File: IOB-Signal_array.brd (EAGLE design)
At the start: 106.7 x 104.1 mm, 104 parts

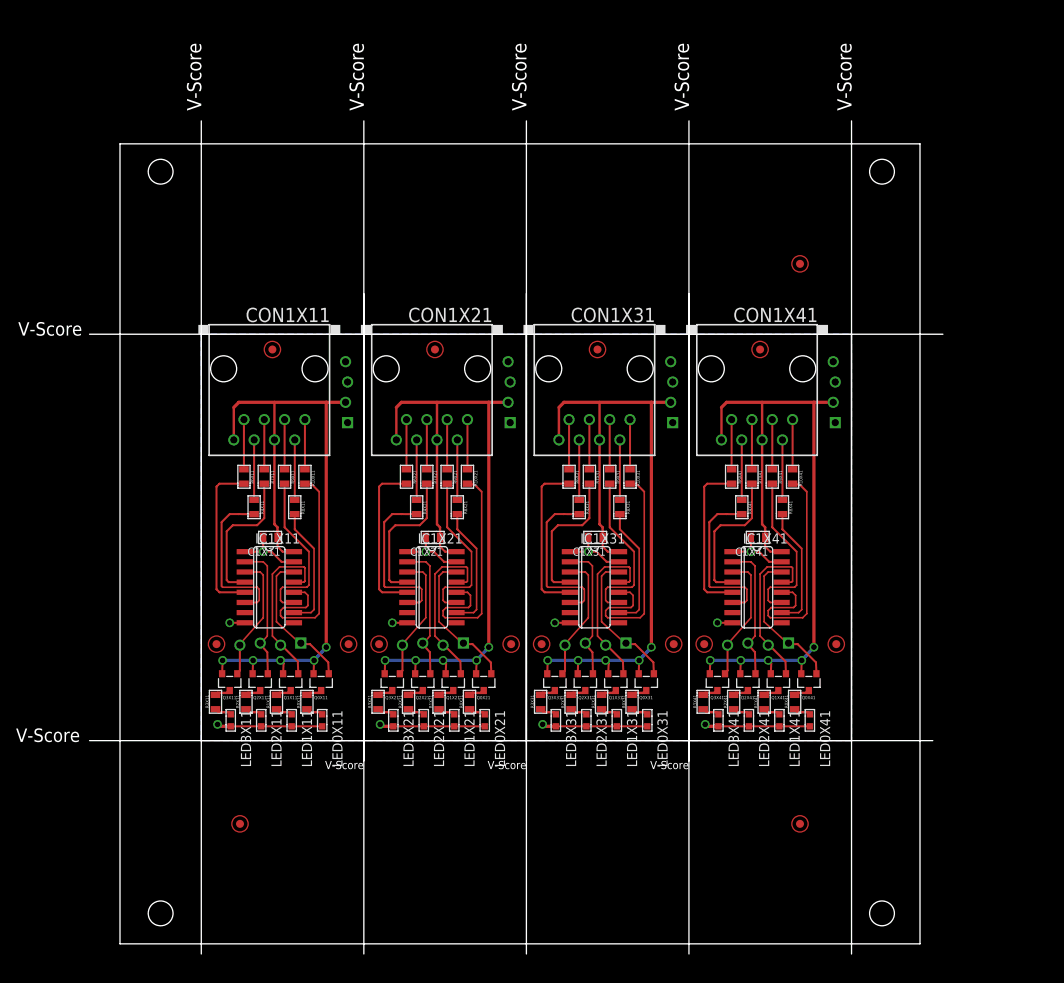
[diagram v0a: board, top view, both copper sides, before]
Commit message: new IOB format
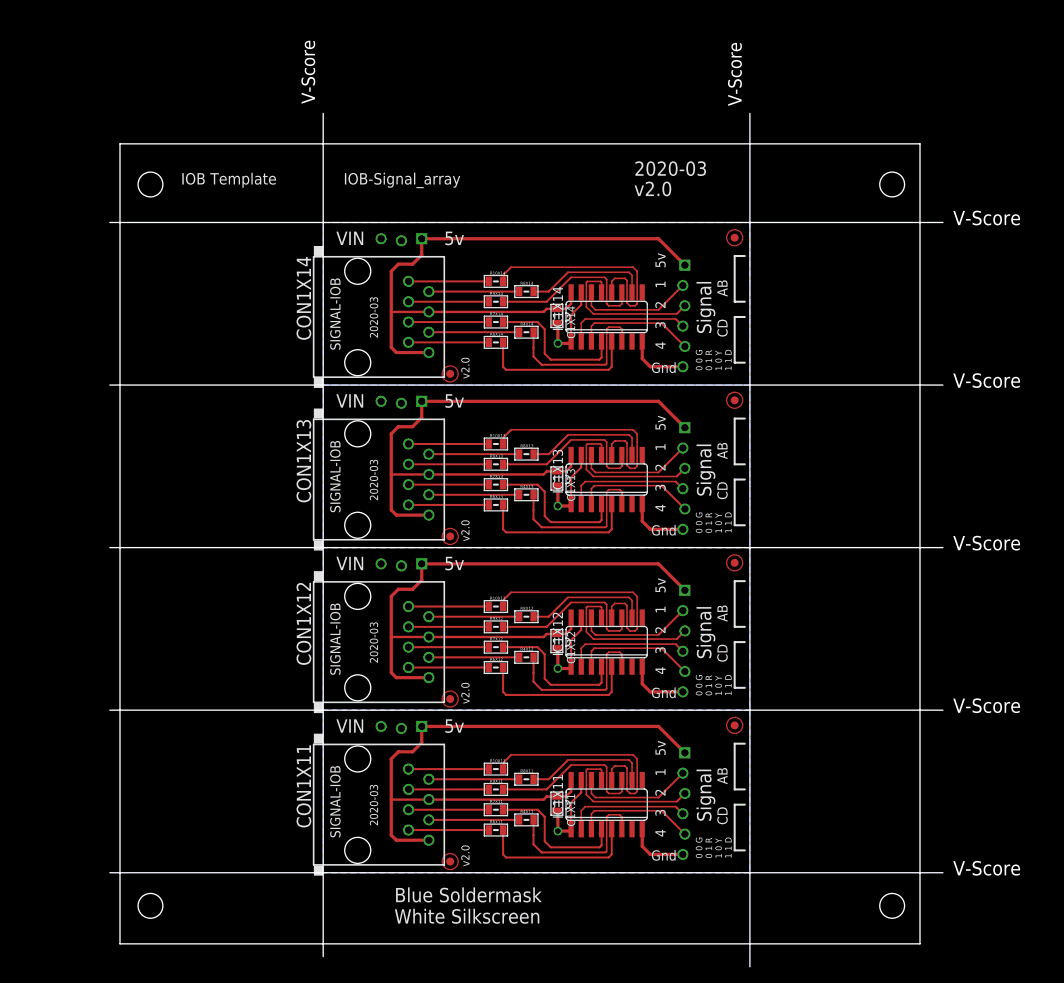
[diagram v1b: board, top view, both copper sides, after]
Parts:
- removed C1X21, C1X31, C1X41: (no value), SPCoast:0805-CAP
- removed CON1X21, CON1X31, CON1X41: (no value), SPCoast:RJ45-NO-SHIELD
- removed FID1X21, FID1X31, FID1X41, FID2X11, FID2X21, FID2X31, FID2X41, FID3X21, FID3X31, FID3X41, R8X2, R8X3, R8X4: (no value), SPCoast:FIDUCIAL_1MM
- removed IC1X21, IC1X31, IC1X41: (no value), SPCoast:SO16
- removed IOBX11, IOBX21, IOBX31, IOBX41: (no value), SPCoast:IO4-IOB
- removed LED0X11, LED0X21, LED0X31, LED0X41, LED1X11, LED1X21, LED1X31, LED1X41, LED2X11, LED2X21, LED2X31, LED2X41, LED3X11, LED3X21, LED3X31, LED3X41: (no value), SPCoast:0603-LED
- removed Q0X11, Q0X21, Q0X31, Q0X41, Q1X11, Q1X21, Q1X31, Q1X41, Q2X11, Q2X21, Q2X31, Q2X41, Q3X11, Q3X21, Q3X31, Q3X41: (no value), SPCoast:SOT23-3
- removed R0X11, R0X21, R0X31, R0X41, R10X21, R10X31, R10X41, R1X11, R1X21, R1X31, R1X41, R2X11, R2X21, R2X31, R2X41, R3X11, R3X21, R3X31, R3X41, R4X21, R4X31, R4X41, R6X21, R6X31, R6X41, R7X21, R7X31, R7X41, R8X21, R8X31, R8X41, R9X21, R9X31, R9X41: (no value), SPCoast:0805-RES
- removed R8X1: (no value), SPCoast:BOARD-DINRAIL-3.17IN-4X-IOB
- added C1X12, C1X13, C1X14: (no value), SPCoast:0805-CAP
- added CON1X12, CON1X13, CON1X14: (no value), SPCoast:RJ45-NO-SHIELD
- added FID1X12, FID1X13, FID1X14, FID3X12, FID3X13, FID3X14: (no value), SPCoast:FIDUCIAL_1MM
- added IC1X12, IC1X13, IC1X14: (no value), SPCoast:SO16
- added R10X12, R10X13, R10X14, R4X12, R4X13, R4X14, R6X12, R6X13, R6X14, R7X12, R7X13, R7X14, R8X12, R8X13, R8X14, R9X12, R9X13, R9X14: (no value), SPCoast:0805-RES
- added U$1X1: (no value), SPCoast:BOARD-DINRAIL-3.17IN-H4X-IOB
- added U$1X11, U$1X12, U$1X13, U$1X14: (no value), SPCoast:IO4-IOB
- moved FID1X11 67.8 mm to (41.3, 10.3), turned to 0 degrees
- moved CON1X11 55.6 mm to (29.7, 17.4), turned to 270 degrees
- moved R6X11 54.3 mm to (47.0, 14.2), turned to 0 degrees
- moved R4X11 51.9 mm to (50.8, 15.5), turned to 0 degrees
- moved R7X11 50.7 mm to (47.0, 16.8), turned to 0 degrees
- moved IC1X11 50.2 mm to (60.8, 17.4), turned to 0 degrees
- moved FID3X11 49.3 mm to (76.8, 27.3), turned to 0 degrees
- moved C1X11 48.9 mm to (54.6, 17.5), turned to 270 degrees
- moved R9X11 47.2 mm to (47.0, 19.3), turned to 0 degrees
- moved R8X11 44.7 mm to (50.8, 20.6), turned to 0 degrees
- moved R10X11 43.7 mm to (47.0, 21.8), turned to 0 degrees
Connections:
- removed net G1-LEDX21: CON1X21.1, R10X21.1
- removed net G1-LEDX31: CON1X31.1, R10X31.1
- removed net G1-LEDX41: CON1X41.1, R10X41.1
- removed net G1X21: IC1X21.12, R10X21.2
- removed net G1X31: IC1X31.12, R10X31.2
- removed net G1X41: IC1X41.12, R10X41.2
- removed net G2-LEDX21: CON1X21.5, R7X21.1
- removed net G2-LEDX31: CON1X31.5, R7X31.1
- removed net G2-LEDX41: CON1X41.5, R7X41.1
- removed net G2X21: IC1X21.4, R7X21.2
- removed net G2X31: IC1X31.4, R7X31.2
- removed net G2X41: IC1X41.4, R7X41.2
- removed net GNDX21: C1X21.2, IC1X21.1, IC1X21.15, IC1X21.8, IOBX21.G@1, IOBX21.G@2, LED0X21.C, LED1X21.C, LED2X21.C, LED3X21.C
- removed net GNDX31: C1X31.2, IC1X31.1, IC1X31.15, IC1X31.8, IOBX31.G@1, IOBX31.G@2, LED0X31.C, LED1X31.C, LED2X31.C, LED3X31.C
- removed net GNDX41: C1X41.2, IC1X41.1, IC1X41.15, IC1X41.8, IOBX41.G@1, IOBX41.G@2, LED0X41.C, LED1X41.C, LED2X41.C, LED3X41.C
- removed net N$11X11: Q0X11.3, R0X11.2
- removed net N$11X21: Q0X21.3, R0X21.2
- removed net N$11X31: Q0X31.3, R0X31.2
- removed net N$11X41: Q0X41.3, R0X41.2
- removed net N$2X11: LED0X11.A, R0X11.1
- removed net N$2X21: LED0X21.A, R0X21.1
- removed net N$2X31: LED0X31.A, R0X31.1
- removed net N$2X41: LED0X41.A, R0X41.1
- removed net N$30X11: Q1X11.3, R1X11.2
- removed net N$30X21: Q1X21.3, R1X21.2
- removed net N$30X31: Q1X31.3, R1X31.2
- removed net N$30X41: Q1X41.3, R1X41.2
- removed net N$31X11: Q2X11.3, R2X11.2
- removed net N$31X21: Q2X21.3, R2X21.2
- removed net N$31X31: Q2X31.3, R2X31.2
- removed net N$31X41: Q2X41.3, R2X41.2
- removed net N$32X11: Q3X11.3, R3X11.2
- removed net N$32X21: Q3X21.3, R3X21.2
- removed net N$32X31: Q3X31.3, R3X31.2
- removed net N$32X41: Q3X41.3, R3X41.2
- removed net N$3X11: LED1X11.A, R1X11.1
- removed net N$3X21: LED1X21.A, R1X21.1
- removed net N$3X31: LED1X31.A, R1X31.1
- removed net N$3X41: LED1X41.A, R1X41.1
- removed net N$4X11: LED2X11.A, R2X11.1
- removed net N$4X21: LED2X21.A, R2X21.1
- removed net N$4X31: LED2X31.A, R2X31.1
- removed net N$4X41: LED2X41.A, R2X41.1
- removed net N$5X11: LED3X11.A, R3X11.1
- removed net N$5X21: LED3X21.A, R3X21.1
- removed net N$5X31: LED3X31.A, R3X31.1
- removed net N$5X41: LED3X41.A, R3X41.1
- removed net P1X21: IC1X21.14, IOBX21.P1, Q0X21.1
- removed net P1X31: IC1X31.14, IOBX31.P1, Q0X31.1
- removed net P1X41: IC1X41.14, IOBX41.P1, Q0X41.1
- removed net P2X21: IC1X21.13, IOBX21.P2, Q1X21.1
- removed net P2X31: IC1X31.13, IOBX31.P2, Q1X31.1
- removed net P2X41: IC1X41.13, IOBX41.P2, Q1X41.1
- removed net P3X21: IC1X21.2, IOBX21.P3, Q2X21.1
- removed net P3X31: IC1X31.2, IOBX31.P3, Q2X31.1
- removed net P3X41: IC1X41.2, IOBX41.P3, Q2X41.1
- removed net P4X21: IC1X21.3, IOBX21.P4, Q3X21.1
- removed net P4X31: IC1X31.3, IOBX31.P4, Q3X31.1
- removed net P4X41: IC1X41.3, IOBX41.P4, Q3X41.1
- removed net R1-LEDX21: CON1X21.3, R9X21.1
- removed net R1-LEDX31: CON1X31.3, R9X31.1
- removed net R1-LEDX41: CON1X41.3, R9X41.1
- removed net R1X21: IC1X21.11, R9X21.2
- removed net R1X31: IC1X31.11, R9X31.2
- removed net R1X41: IC1X41.11, R9X41.2
- removed net R2-LEDX21: CON1X21.7, R6X21.1
- removed net R2-LEDX31: CON1X31.7, R6X31.1
- removed net R2-LEDX41: CON1X41.7, R6X41.1
- removed net R2X21: IC1X21.5, R6X21.2
- removed net R2X31: IC1X31.5, R6X31.2
- removed net R2X41: IC1X41.5, R6X41.2
- removed net VCCIOX21: IOBX21.V+
- removed net VCCIOX31: IOBX31.V+
- removed net VCCIOX41: IOBX41.V+
- removed net VCCX21: C1X21.1, CON1X21.4, CON1X21.8, IC1X21.16, IOBX21.V5, Q0X21.2, Q1X21.2, Q2X21.2, Q3X21.2
- removed net VCCX31: C1X31.1, CON1X31.4, CON1X31.8, IC1X31.16, IOBX31.V5, Q0X31.2, Q1X31.2, Q2X31.2, Q3X31.2
- removed net VCCX41: C1X41.1, CON1X41.4, CON1X41.8, IC1X41.16, IOBX41.V5, Q0X41.2, Q1X41.2, Q2X41.2, Q3X41.2
- removed net Y1-LEDX21: CON1X21.2, R8X21.1
- removed net Y1-LEDX31: CON1X31.2, R8X31.1
- removed net Y1-LEDX41: CON1X41.2, R8X41.1
- removed net Y1X21: IC1X21.10, R8X21.2
- removed net Y1X31: IC1X31.10, R8X31.2
- removed net Y1X41: IC1X41.10, R8X41.2
- removed net Y2-LEDX21: CON1X21.6, R4X21.1
- removed net Y2-LEDX31: CON1X31.6, R4X31.1
- removed net Y2-LEDX41: CON1X41.6, R4X41.1
- removed net Y2X21: IC1X21.6, R4X21.2
- removed net Y2X31: IC1X31.6, R4X31.2
- removed net Y2X41: IC1X41.6, R4X41.2
- new net G1-LEDX12: CON1X12.1, R10X12.1
- new net G1-LEDX13: CON1X13.1, R10X13.1
- new net G1-LEDX14: CON1X14.1, R10X14.1
- new net G1X12: IC1X12.12, R10X12.2
- new net G1X13: IC1X13.12, R10X13.2
- new net G1X14: IC1X14.12, R10X14.2
- new net G2-LEDX12: CON1X12.5, R7X12.1
- new net G2-LEDX13: CON1X13.5, R7X13.1
- new net G2-LEDX14: CON1X14.5, R7X14.1
- new net G2X12: IC1X12.4, R7X12.2
- new net G2X13: IC1X13.4, R7X13.2
- new net G2X14: IC1X14.4, R7X14.2
- new net GNDX12: C1X12.2, IC1X12.1, IC1X12.15, IC1X12.8, U$1X12.G@3
- new net GNDX13: C1X13.2, IC1X13.1, IC1X13.15, IC1X13.8, U$1X13.G@3
- new net GNDX14: C1X14.2, IC1X14.1, IC1X14.15, IC1X14.8, U$1X14.G@3
- new net P1X12: IC1X12.14, U$1X12.P1
- new net P1X13: IC1X13.14, U$1X13.P1
- new net P1X14: IC1X14.14, U$1X14.P1
- new net P2X12: IC1X12.13, U$1X12.P2
- new net P2X13: IC1X13.13, U$1X13.P2
- new net P2X14: IC1X14.13, U$1X14.P2
- new net P3X12: IC1X12.2, U$1X12.P3
- new net P3X13: IC1X13.2, U$1X13.P3
- new net P3X14: IC1X14.2, U$1X14.P3
- new net P4X12: IC1X12.3, U$1X12.P4
- new net P4X13: IC1X13.3, U$1X13.P4
- new net P4X14: IC1X14.3, U$1X14.P4
- new net R1-LEDX12: CON1X12.3, R9X12.1
- new net R1-LEDX13: CON1X13.3, R9X13.1
- new net R1-LEDX14: CON1X14.3, R9X14.1
- new net R1X12: IC1X12.11, R9X12.2
- new net R1X13: IC1X13.11, R9X13.2
- new net R1X14: IC1X14.11, R9X14.2
- new net R2-LEDX12: CON1X12.7, R6X12.1
- new net R2-LEDX13: CON1X13.7, R6X13.1
- new net R2-LEDX14: CON1X14.7, R6X14.1
- new net R2X12: IC1X12.5, R6X12.2
- new net R2X13: IC1X13.5, R6X13.2
- new net R2X14: IC1X14.5, R6X14.2
- new net VCCIOX12: U$1X12.V+
- new net VCCIOX13: U$1X13.V+
- new net VCCIOX14: U$1X14.V+
- new net VCCX12: C1X12.1, CON1X12.4, CON1X12.8, IC1X12.16, U$1X12.V5, U$1X12.V5@1
- new net VCCX13: C1X13.1, CON1X13.4, CON1X13.8, IC1X13.16, U$1X13.V5, U$1X13.V5@1
- new net VCCX14: C1X14.1, CON1X14.4, CON1X14.8, IC1X14.16, U$1X14.V5, U$1X14.V5@1
- new net Y1-LEDX12: CON1X12.2, R8X12.1
- new net Y1-LEDX13: CON1X13.2, R8X13.1
- new net Y1-LEDX14: CON1X14.2, R8X14.1
- new net Y1X12: IC1X12.10, R8X12.2
- new net Y1X13: IC1X13.10, R8X13.2
- new net Y1X14: IC1X14.10, R8X14.2
- new net Y2-LEDX12: CON1X12.6, R4X12.1
- new net Y2-LEDX13: CON1X13.6, R4X13.1
- new net Y2-LEDX14: CON1X14.6, R4X14.1
- new net Y2X12: IC1X12.6, R4X12.2
- new net Y2X13: IC1X13.6, R4X13.2
- new net Y2X14: IC1X14.6, R4X14.2
- net GNDX11: now also U$1X11.G@3; no longer IOBX11.G@1, IOBX11.G@2, LED0X11.C, LED1X11.C, LED2X11.C, LED3X11.C
- net P1X11: now also U$1X11.P1; no longer IOBX11.P1, Q0X11.1
- net P2X11: now also U$1X11.P2; no longer IOBX11.P2, Q1X11.1
- net P3X11: now also U$1X11.P3; no longer IOBX11.P3, Q2X11.1
- net P4X11: now also U$1X11.P4; no longer IOBX11.P4, Q3X11.1
- net VCCIOX11: now also U$1X11.V+; no longer IOBX11.V+
- net VCCX11: now also U$1X11.V5, U$1X11.V5@1; no longer IOBX11.V5, Q0X11.2, Q1X11.2, Q2X11.2, Q3X11.2
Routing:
- net VCCX41: track 90.1 -> 0.00 mm, vias 5 -> 0
- net VCCX31: track 90.1 -> 0.00 mm, vias 5 -> 0
- net VCCX21: track 90.1 -> 0.00 mm, vias 5 -> 0
- net VCCX14: track 0.00 -> 79.8 mm
- net VCCX13: track 0.00 -> 79.8 mm
- net VCCX12: track 0.00 -> 79.8 mm
- net G1X41: track 30.0 -> 0.00 mm
- net G1X21: track 30.0 -> 0.00 mm
- net G1X31: track 30.0 -> 0.00 mm
- net G1X13: track 0.00 -> 30.0 mm
- net G1X12: track 0.00 -> 30.0 mm
- net G1X14: track 0.00 -> 30.0 mm
- net GNDX41: track 23.5 -> 0.00 mm, vias 3 -> 0
- net GNDX21: track 23.5 -> 0.00 mm, vias 3 -> 0
- net GNDX31: track 23.5 -> 0.00 mm, vias 3 -> 0
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- added copper zone on layer 16, net GNDX12
- added copper zone on layer 16, net GNDX13
- added copper zone on layer 16, net GNDX14
- removed copper zone on layer 16, net GNDX21
- removed copper zone on layer 16, net GNDX31
- removed copper zone on layer 16, net GNDX41
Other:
- board size 106.7 x 104.1 mm -> 104.1 x 106.7 mm
- board text added: "2020-03"
- board text added: "AB"
- board text added: "Blue Soldermask White Silkscreen"
- board text added: "C1"
- board text added: "CD"
- board text added: "CON1"
- board text added: "IC1"
- board text added: "R10"
- board text added: "R4"
- board text added: "R6"
- board text added: "R7"
- board text added: "R8"
- board text added: "R9"
- board text added: "SIGNAL-IOB"
- board text added: "v2.0"
- board text removed: "(15,15)"
- board text removed: "(15,85)"
- board text removed: "(85,85)"
- board text removed: "2019-11"
- board text removed: "Black Soldermask, White Silkscreen"
- board text removed: "IO Interface"
- board text removed: "IO4-IOB"
- board text removed: "IOB Signal Driver"
- board text removed: "Made in the PCR, Coast Div, NMRA"
- board text removed: "Model Railroading is Fun!"
- board text removed: "V-Score"
- board text removed: "V1.1"
- board text removed: "v1.1"
